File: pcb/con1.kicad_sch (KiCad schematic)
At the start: 16 parts, among them J7 DIN41612_02x32_AC, U6 M24C02-WMN, U7 USBLC6-2SC6

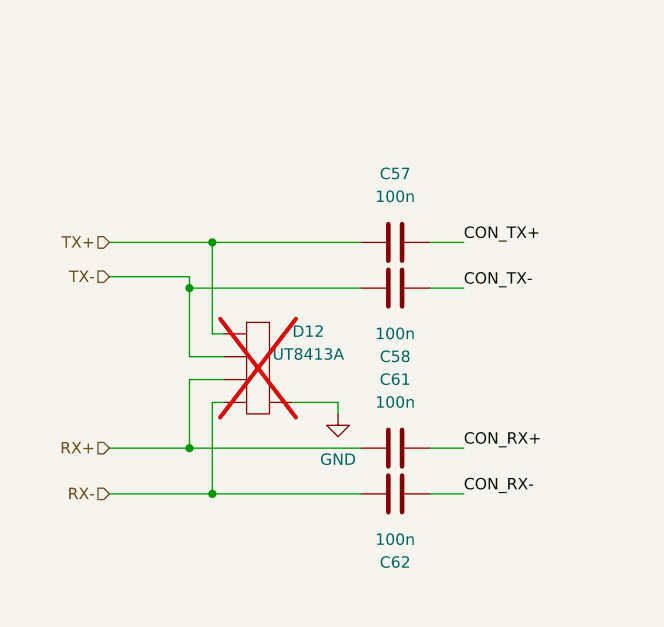
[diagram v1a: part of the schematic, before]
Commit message: More routing
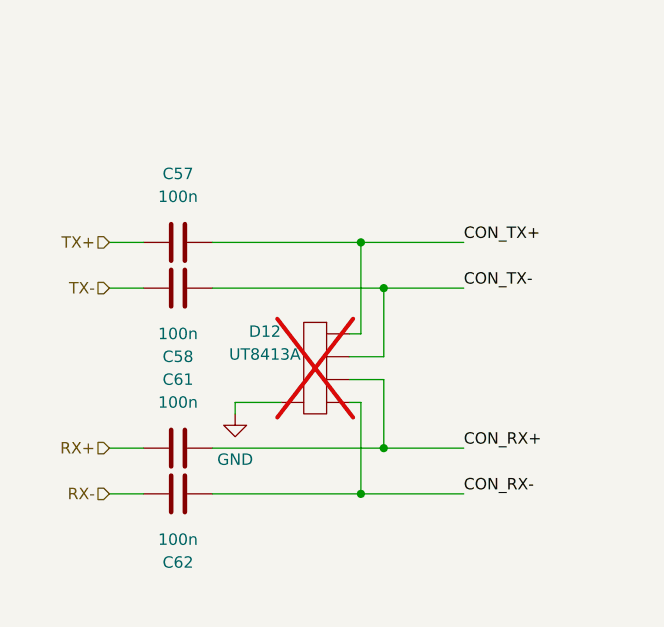
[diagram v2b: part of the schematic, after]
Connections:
- net CON_RX+: now also C61.2, D12.2, D12.9; no longer C61.1
- net CON_RX-: now also C62.2, D12.1, D12.10; no longer C62.1
- net CON_TX+: now also C57.2, D12.5, D12.6; no longer C57.1
- net CON_TX-: now also C58.2, D12.4, D12.7; no longer C58.1
- net RX+: now also C61.1; no longer C61.2, D12.2, D12.9
- net RX-: now also C62.1; no longer C62.2, D12.1, D12.10
- net TX+: now also C57.1; no longer C57.2, D12.5, D12.6
- net TX-: now also C58.1; no longer C58.2, D12.4, D12.7
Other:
- moved on the sheet: C57, C58, C61, C62, D12
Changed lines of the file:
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@@
 	)
 	(junction
-		(at 104.14 114.3)
+		(at 125.73 114.3)
 		(diameter 0)
 		(color 0 0 0 0)
@@
 	)
 	(junction
-		(at 106.68 119.38)
+		(at 123.19 119.38)
 		(diameter 0)
 		(color 0 0 0 0)
@@
 	)
 	(junction
-		(at 104.14 96.52)
+		(at 125.73 96.52)
 		(diameter 0)
 		(color 0 0 0 0)
@@
 	)
 	(junction
-		(at 106.68 91.44)
+		(at 123.19 91.44)
 		(diameter 0)
 		(color 0 0 0 0)
@@
 	(wire
 		(pts
-			(xy 106.68 119.38) (xy 123.19 119.38)
+			(xy 123.19 119.38) (xy 106.68 119.38)
 		)
 		(stroke
@@
 	(wire
 		(pts
-			(xy 95.25 119.38) (xy 106.68 119.38)
+			(xy 134.62 119.38) (xy 123.19 119.38)
 		)
 		(stroke
@@
 	(wire
 		(pts
-			(xy 107.95 106.68) (xy 104.14 106.68)
+			(xy 121.92 106.68) (xy 125.73 106.68)
 		)
 		(stroke
@@
 	(wire
 		(pts
-			(xy 120.65 109.22) (xy 120.65 110.49)
+			(xy 109.22 109.22) (xy 109.22 110.49)
 		)
 		(stroke
@@
 	(wire
 		(pts
-			(xy 134.62 114.3) (xy 130.81 114.3)
+			(xy 95.25 114.3) (xy 99.06 114.3)
 		)
 		(stroke
@@
 	(wire
 		(pts
-			(xy 107.95 109.22) (xy 106.68 109.22)
+			(xy 121.92 109.22) (xy 123.19 109.22)
 		)
 		(stroke
@@
 	(wire
 		(pts
-			(xy 134.62 91.44) (xy 130.81 91.44)
+			(xy 95.25 91.44) (xy 99.06 91.44)
 		)
 		(stroke
@@
 	(wire
 		(pts
-			(xy 95.25 91.44) (xy 106.68 91.44)
+			(xy 134.62 91.44) (xy 123.19 91.44)
 		)
 		(stroke
@@
 	(wire
 		(pts
-			(xy 107.95 104.14) (xy 104.14 104.14)
+			(xy 121.92 104.14) (xy 125.73 104.14)
 		)
 		(stroke
@@
 	(wire
 		(pts
-			(xy 95.25 114.3) (xy 104.14 114.3)
+			(xy 134.62 114.3) (xy 125.73 114.3)
 		)
 		(stroke
@@
 	(wire
 		(pts
-			(xy 134.62 96.52) (xy 130.81 96.52)
+			(xy 95.25 96.52) (xy 99.06 96.52)
 		)
 		(stroke
@@
 	(wire
 		(pts
-			(xy 104.14 96.52) (xy 123.19 96.52)
+			(xy 125.73 96.52) (xy 106.68 96.52)
 		)
 		(stroke
@@
 	(wire
 		(pts
-			(xy 106.68 109.22) (xy 106.68 119.38)
+			(xy 123.19 109.22) (xy 123.19 119.38)
 		)
 		(stroke
@@
 	(wire
 		(pts
-			(xy 115.57 109.22) (xy 120.65 109.22)
+			(xy 114.3 109.22) (xy 109.22 109.22)
 		)
 		(stroke
@@
 	(wire
 		(pts
-			(xy 104.14 96.52) (xy 104.14 104.14)
+			(xy 125.73 96.52) (xy 125.73 104.14)
 		)
 		(stroke
@@
 	(wire
 		(pts
-			(xy 106.68 91.44) (xy 123.19 91.44)
+			(xy 123.19 91.44) (xy 106.68 91.44)
 		)
 		(stroke
@@
 	(wire
 		(pts
-			(xy 106.68 91.44) (xy 106.68 101.6)
+			(xy 123.19 91.44) (xy 123.19 101.6)
 		)
 		(stroke
@@
 	(wire
 		(pts
-			(xy 104.14 114.3) (xy 123.19 114.3)
+			(xy 125.73 114.3) (xy 106.68 114.3)
 		)
 		(stroke
@@
 	(wire
 		(pts
-			(xy 107.95 101.6) (xy 106.68 101.6)
+			(xy 121.92 101.6) (xy 123.19 101.6)
 		)
 		(stroke
@@
 	(wire
 		(pts
-			(xy 134.62 119.38) (xy 130.81 119.38)
+			(xy 95.25 119.38) (xy 99.06 119.38)
 		)
 		(stroke
@@
 	(wire
 		(pts
-			(xy 104.14 95.25) (xy 104.14 96.52)
-		)
-		(stroke
-			(width 0)
-			(type default)
-		)
-	)
-	(wire
-		(pts
-			(xy 95.25 95.25) (xy 104.14 95.25)
+			(xy 134.62 96.52) (xy 125.73 96.52)
 		)
 		(stroke
@@
 	(wire
 		(pts
-			(xy 104.14 106.68) (xy 104.14 114.3)
+			(xy 125.73 106.68) (xy 125.73 114.3)
 		)
 		(stroke
@@
 	(hierarchical_label "TX-"
 		(shape input)
-		(at 95.25 95.25 180)
+		(at 95.25 96.52 180)
 		(effects
 			(font
@@
 	(symbol
 		(lib_id "Device:C")
-		(at 127 91.44 270)
+		(at 102.87 91.44 90)
+		(mirror x)
 		(unit 1)
 		(body_style 1)
@@
 		(fields_autoplaced yes)
 		(property "Reference" "C57"
-			(at 127 83.82 90)
+			(at 102.87 83.82 90)
 			(show_name no)
 			(do_not_autoplace no)
@@
 		)
 		(property "Value" "100n"
-			(at 127 86.36 90)
+			(at 102.87 86.36 90)
 			(show_name no)
 			(do_not_autoplace no)
@@
 		)
 		(property "Footprint" "Capacitor_SMD:C_0805_2012Metric"
-			(at 123.19 92.4052 0)
+			(at 106.68 92.4052 0)
 			(hide yes)
 			(show_name no)
@@
 		)
 		(property "Datasheet" ""
-			(at 127 91.44 0)
+			(at 102.87 91.44 0)
 			(hide yes)
 			(show_name no)
@@
 		)
 		(property "Description" "CGA4J3X7T2E104KAA"
-			(at 127 91.44 0)
+			(at 102.87 91.44 0)
 			(hide yes)
 			(show_name no)
@@
 	(symbol
 		(lib_id "Device:C")
-		(at 127 96.52 270)
-		(mirror x)
+		(at 102.87 96.52 90)
 		(unit 1)
 		(body_style 1)
@@
 		(fields_autoplaced yes)
 		(property "Reference" "C58"
-			(at 127 104.14 90)
+			(at 102.87 104.14 90)
 			(show_name no)
 			(do_not_autoplace no)
@@
 		)
 		(property "Value" "100n"
-			(at 127 101.6 90)
+			(at 102.87 101.6 90)
 			(show_name no)
 			(do_not_autoplace no)
@@
 		)
 		(property "Footprint" "Capacitor_SMD:C_0805_2012Metric"
-			(at 123.19 95.5548 0)
+			(at 106.68 95.5548 0)
 			(hide yes)
 			(show_name no)
@@
 		)
 		(property "Datasheet" ""
-			(at 127 96.52 0)
+			(at 102.87 96.52 0)
 			(hide yes)
 			(show_name no)
@@
 		)
 		(property "Description" "CGA4J3X7T2E104KAA"
-			(at 127 96.52 0)
+			(at 102.87 96.52 0)
 			(hide yes)
 			(show_name no)
@@
 	(symbol
 		(lib_id "Device:C")
-		(at 127 119.38 270)
-		(mirror x)
+		(at 102.87 119.38 90)
 		(unit 1)
 		(body_style 1)
@@
 		(fields_autoplaced yes)
 		(property "Reference" "C62"
-			(at 127 127 90)
+			(at 102.87 127 90)
 			(show_name no)
 			(do_not_autoplace no)
@@
 		)
 		(property "Value" "100n"
-			(at 127 124.46 90)
+			(at 102.87 124.46 90)
 			(show_name no)
 			(do_not_autoplace no)
@@
 		)
 		(property "Footprint" "Capacitor_SMD:C_0805_2012Metric"
-			(at 123.19 118.4148 0)
+			(at 106.68 118.4148 0)
 			(hide yes)
 			(show_name no)
@@
 		)
 		(property "Datasheet" ""
-			(at 127 119.38 0)
+			(at 102.87 119.38 0)
 			(hide yes)
 			(show_name no)
@@
 		)
 		(property "Description" "CGA4J3X7T2E104KAA"
-			(at 127 119.38 0)
+			(at 102.87 119.38 0)
 			(hide yes)
 			(show_name no)
@@
 	(symbol
 		(lib_id "power:GND")
-		(at 120.65 110.49 0)
+		(at 109.22 110.49 0)
+		(mirror y)
 		(unit 1)
 		(body_style 1)
@@
 		(fields_autoplaced yes)
 		(property "Reference" "#PWR061"
-			(at 120.65 116.84 0)
+			(at 109.22 116.84 0)
 			(hide yes)
 			(show_name no)
@@
 		)
 		(property "Value" "GND"
-			(at 120.65 115.57 0)
+			(at 109.22 115.57 0)
 			(show_name no)
 			(do_not_autoplace no)
@@
 		)
 		(property "Footprint" ""
-			(at 120.65 110.49 0)
+			(at 109.22 110.49 0)
 			(hide yes)
 			(show_name no)
@@
 		)
 		(property "Datasheet" ""
-			(at 120.65 110.49 0)
+			(at 109.22 110.49 0)
 			(hide yes)
 			(show_name no)
@@
 		)
 		(property "Description" "Power symbol creates a global label with name \"GND\" , ground"
-			(at 120.65 110.49 0)
+			(at 109.22 110.49 0)
 			(hide yes)
 			(show_name no)
@@
 	(symbol
 		(lib_id "Device:C")
-		(at 127 114.3 270)
+		(at 102.87 114.3 90)
+		(mirror x)
 		(unit 1)
 		(body_style 1)
@@
 		(dnp no)
 		(property "Reference" "C61"
-			(at 127 106.68 90)
+			(at 102.87 106.68 90)
 			(show_name no)
 			(do_not_autoplace no)
@@
 		)
 		(property "Value" "100n"
-			(at 127 109.22 90)
+			(at 102.87 109.22 90)
 			(show_name no)
 			(do_not_autoplace no)
@@
 		)
 		(property "Footprint" "Capacitor_SMD:C_0805_2012Metric"
-			(at 123.19 115.2652 0)
+			(at 106.68 115.2652 0)
 			(hide yes)
 			(show_name no)
@@
 		)
 		(property "Datasheet" ""
-			(at 127 114.3 0)
+			(at 102.87 114.3 0)
 			(hide yes)
 			(show_name no)
@@
 		)
 		(property "Description" "CGA4J3X7T2E104KAA"
-			(at 127 114.3 0)
+			(at 102.87 114.3 0)
 			(hide yes)
 			(show_name no)
@@
 	(symbol
 		(lib_id "Conn:UT8413A")
-		(at 110.49 105.41 0)
+		(at 119.38 105.41 0)
+		(mirror y)
 		(unit 1)
 		(body_style 1)
@@
 		(dnp yes)
 		(property "Reference" "D12"
-			(at 117.348 101.346 0)
+			(at 112.522 101.346 0)
 			(show_name no)
 			(do_not_autoplace no)
@@
 		)
 		(property "Value" "UT8413A"
-			(at 117.348 103.886 0)
+			(at 112.522 103.886 0)
 			(show_name no)
 			(do_not_autoplace no)
@@
 		)
 		(property "Footprint" "Package_DFN_QFN:Diodes_UDFN-10_1.0x2.5mm_P0.5mm"
-			(at 110.49 105.41 0)
+			(at 119.38 105.41 0)
 			(hide yes)
 			(show_name no)
@@
 		)
 		(property "Datasheet" "https://www.tme.eu/Document/2ddf4c2e70778c4b0b01bb008847dce1/UT8413A.pdf"
-			(at 110.49 105.41 0)
+			(at 119.38 105.41 0)
 			(hide yes)
 			(show_name no)
@@
 		)
 		(property "Description" "TRANSIENT VOLTAGE SUPPRESSOR (TVS) ARRAY"
-			(at 110.236 105.664 0)
+			(at 119.634 105.664 0)
 			(hide yes)
 			(show_name no)
@@
 		)
 		(property "Sim.Device" ""
-			(at 110.49 105.41 0)
+			(at 119.38 105.41 0)
 			(hide yes)
 			(show_name no)
@@
 		)
 		(property "Sim.Pins" ""
-			(at 110.49 105.41 0)
+			(at 119.38 105.41 0)
 			(hide yes)
 			(show_name no)
@@
 		)
 		(property "Manufacturer_Part_Number" "UT8413A"
-			(at 110.49 105.41 0)
+			(at 119.38 105.41 0)
 			(hide yes)
 			(show_name no)

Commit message: Add design review docs, expand README, sync PCB routing and production outputs
Routing progress on schematic/PCB, generated production outputs (gerbers,
BOM, PDFs), 3D model cache, and datasheet sync. Adds doc/ (design review
report + TODO) and README overview of architecture/status/repo layout.
Analysis tool output moved to .gitignore (regenerable, not source).
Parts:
- C56, C60: footprint Capacitor_SMD:C_0603_1608Metric_Pad1.08x0.95mm_HandSolder -> Capacitor_SMD:C_0603_1608Metric
- C59: footprint Capacitor_SMD:C_1206_3216Metric_Pad1.33x1.80mm_HandSolder -> Capacitor_SMD:C_1206_3216Metric
- D12: footprint Package_DFN_QFN:Diodes_UDFN-10_1.0x2.5mm_P0.5mm -> Package_DFN_QFN:Diodes_UDFN-10_1x2.5mm_P0.5mm
- R59, R60: footprint Resistor_SMD:R_0603_1608Metric_Pad0.98x0.95mm_HandSolder -> Resistor_SMD:R_0603_1608Metric
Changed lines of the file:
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@@
 			)
 		)
-		(property "Footprint" "Capacitor_SMD:C_0603_1608Metric_Pad1.08x0.95mm_HandSolder"
+		(property "Footprint" "Capacitor_SMD:C_0603_1608Metric"
 			(at 189.5348 92.71 0)
 			(hide yes)
@@
 			)
 		)
-		(property "Footprint" "Capacitor_SMD:C_0603_1608Metric_Pad1.08x0.95mm_HandSolder"
+		(property "Footprint" "Capacitor_SMD:C_0603_1608Metric"
 			(at 86.6648 26.67 0)
 			(hide yes)
@@
 			)
 		)
-		(property "Footprint" "Resistor_SMD:R_0603_1608Metric_Pad0.98x0.95mm_HandSolder"
+		(property "Footprint" "Resistor_SMD:R_0603_1608Metric"
 			(at 131.318 30.48 90)
 			(hide yes)
@@
 			)
 		)
-		(property "Footprint" "Resistor_SMD:R_0603_1608Metric_Pad0.98x0.95mm_HandSolder"
+		(property "Footprint" "Resistor_SMD:R_0603_1608Metric"
 			(at 122.428 30.48 90)
 			(hide yes)
@@
 			)
 		)
-		(property "Footprint" "Capacitor_SMD:C_1206_3216Metric_Pad1.33x1.80mm_HandSolder"
+		(property "Footprint" "Capacitor_SMD:C_1206_3216Metric"
 			(at 181.3052 100.33 0)
 			(hide yes)
@@
 			)
 		)
-		(property "Footprint" "Package_DFN_QFN:Diodes_UDFN-10_1.0x2.5mm_P0.5mm"
+		(property "Footprint" "Package_DFN_QFN:Diodes_UDFN-10_1x2.5mm_P0.5mm"
 			(at 119.38 105.41 0)
 			(hide yes)
